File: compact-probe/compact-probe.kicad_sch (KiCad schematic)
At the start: 25 parts, among them IC1 ATA6561-GBQW-N, J1 Conn_01x08_Male, J2 Conn_01x04_Male, J3 Conn_02x05_Odd_Even, J4 Conn_01x01_Female, J5 Conn_01x01_Female, J6 Conn_01x01_Female, J7 Conn_01x01_Female, J8 Conn_01x01_Female, U4 ESP32-C3-WROOM-02-H4, U6 LT1963AxST-3.3

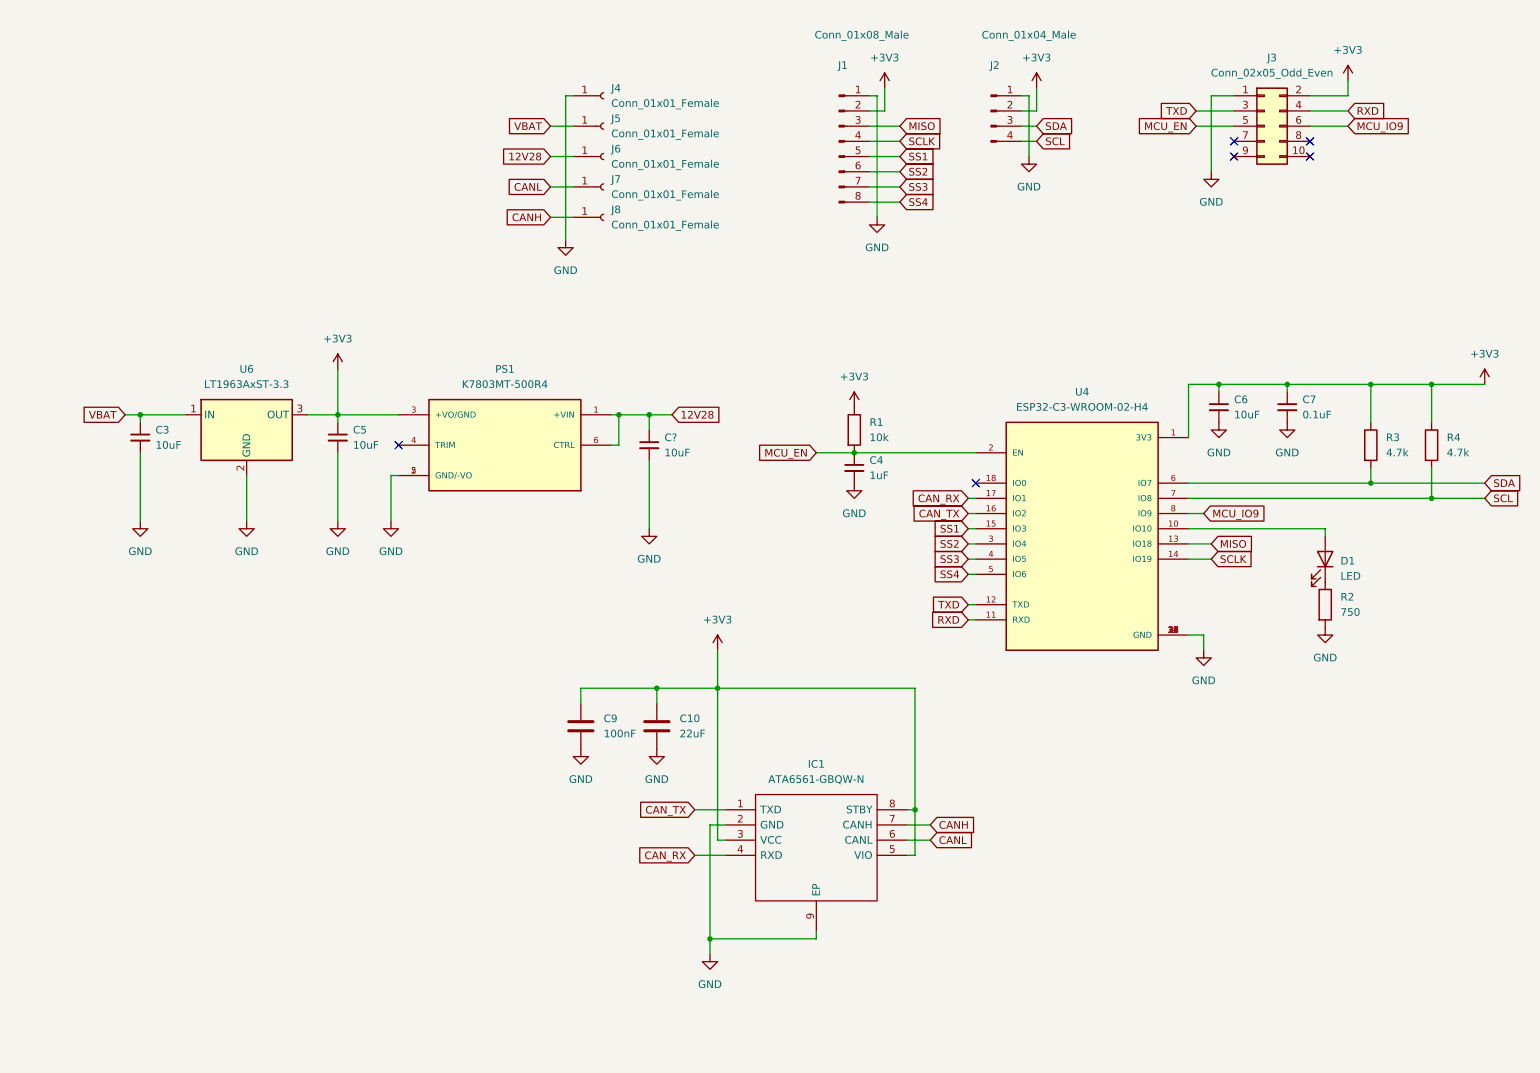
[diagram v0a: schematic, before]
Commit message: Final changes.
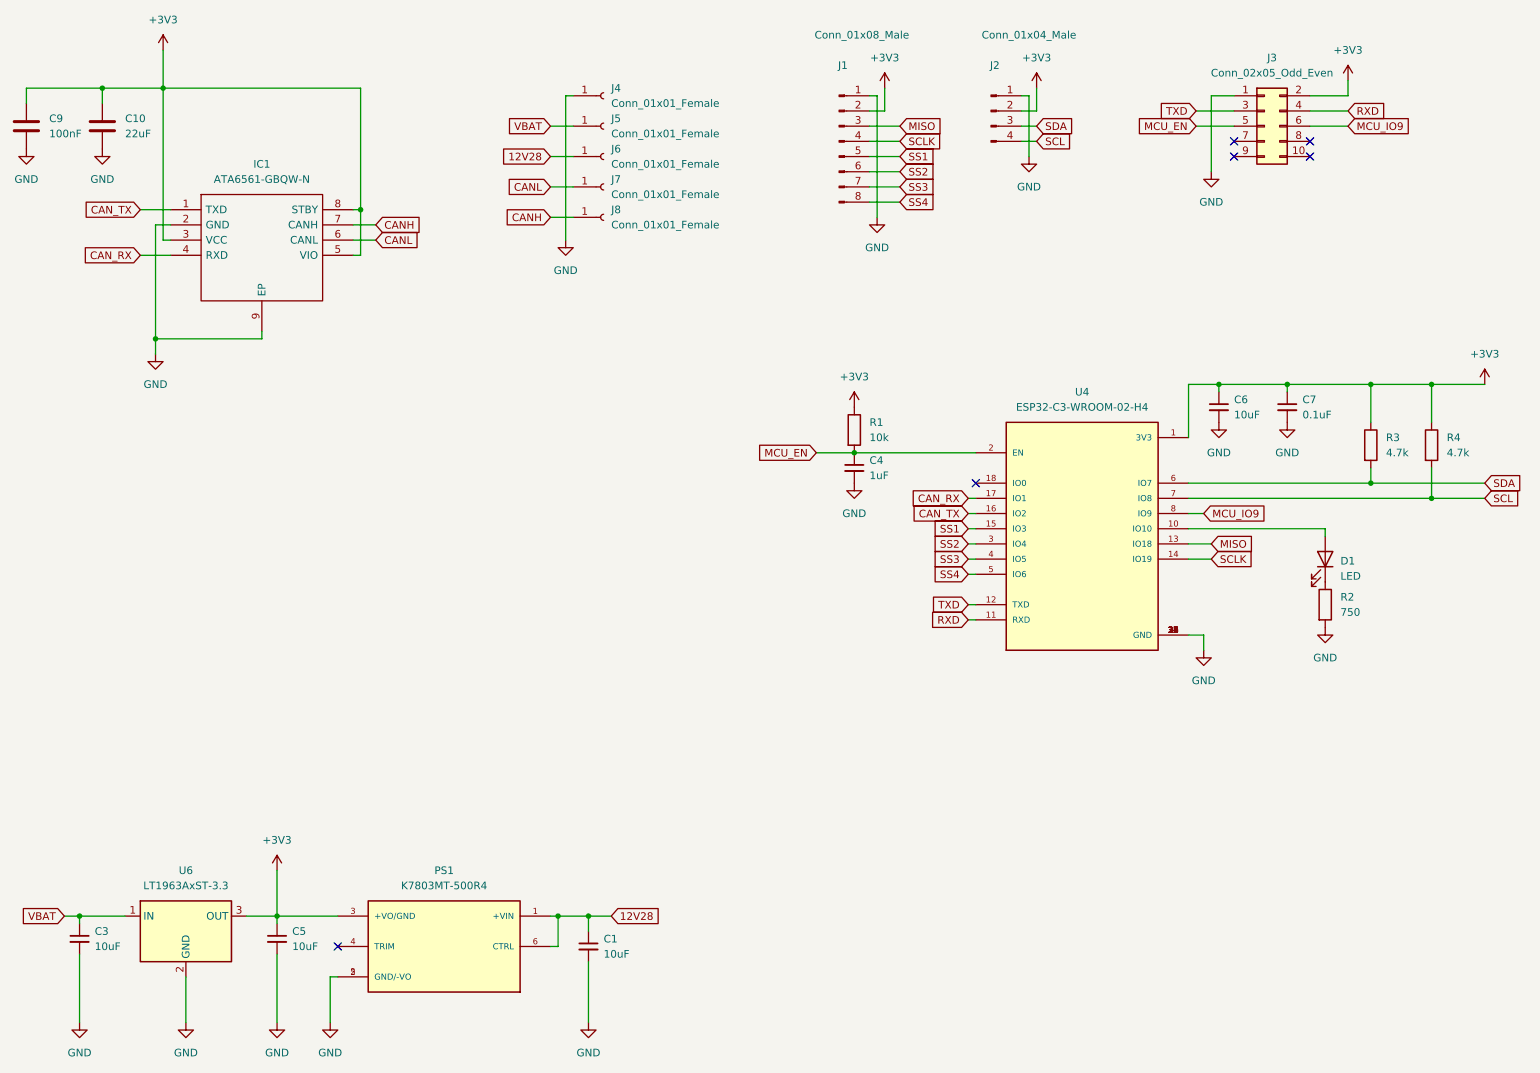
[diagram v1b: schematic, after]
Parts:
- gave numbers to parts that had none: 1
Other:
- moved on the sheet: C1, C10, C3, C5, C9, IC1, PS1, U6
